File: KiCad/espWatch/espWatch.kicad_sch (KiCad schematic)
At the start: 6 parts, among them U1 Level converter, U2 NodeMCU_1.0_(ESP-12E), U3 1.8" TFT ST7735, U4 RTC DS3231

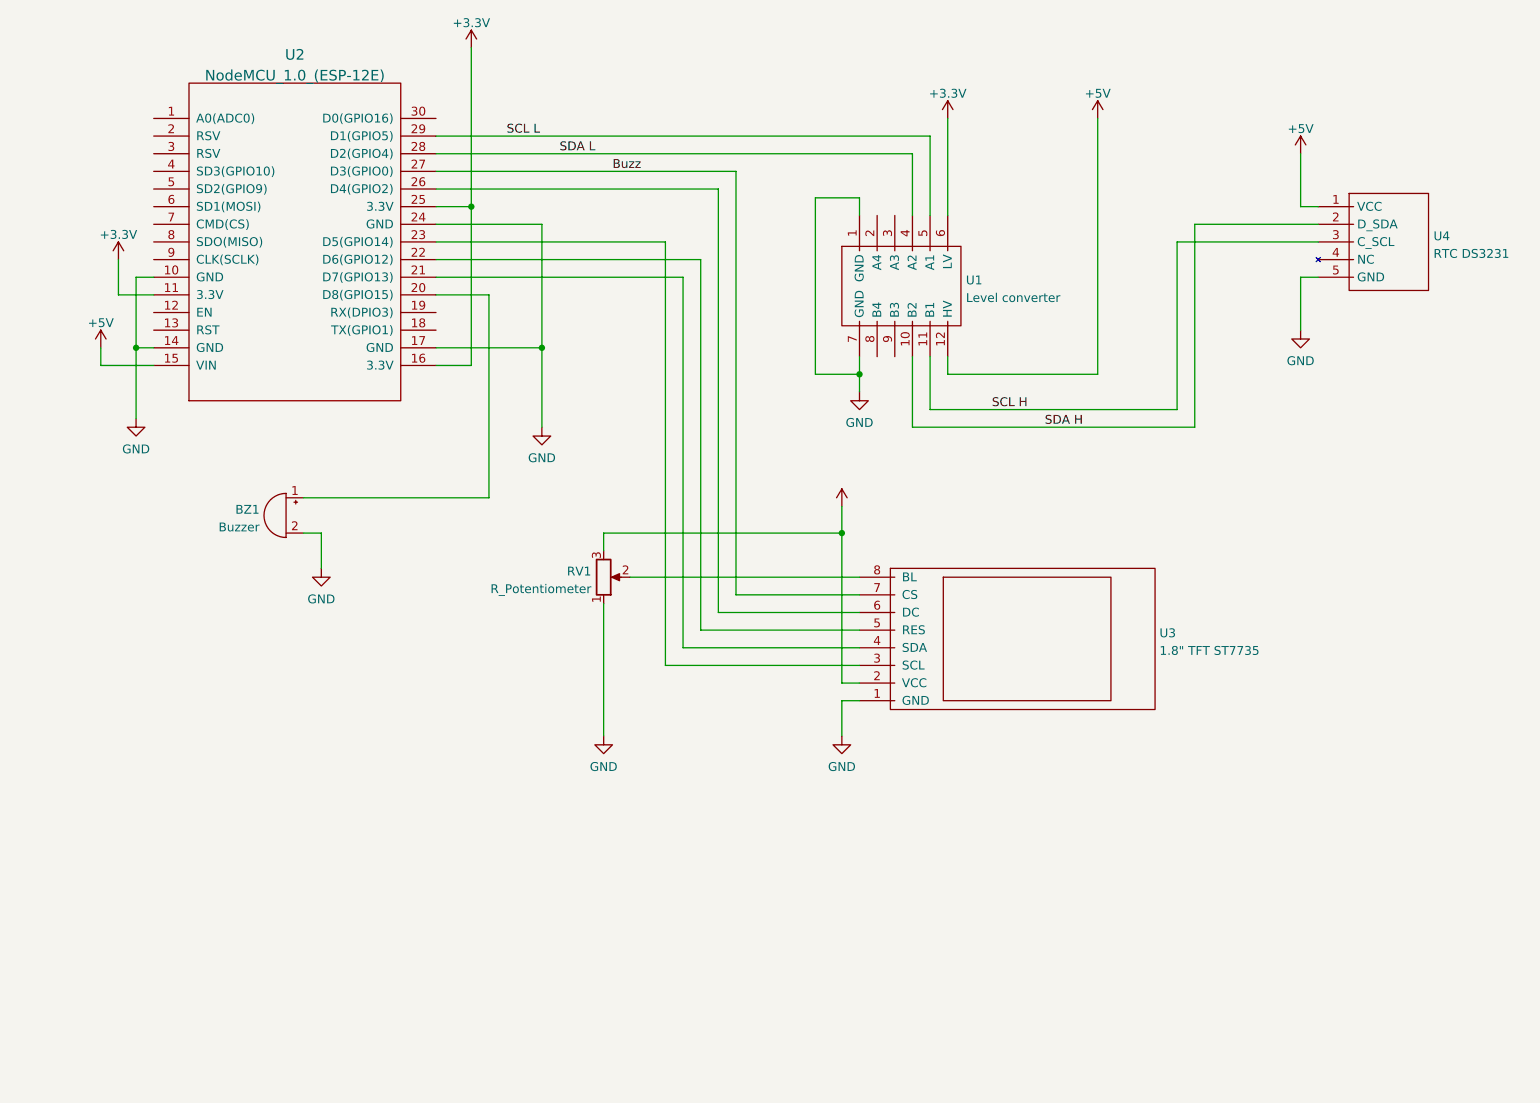
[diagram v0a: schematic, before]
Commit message: pcb and pin config
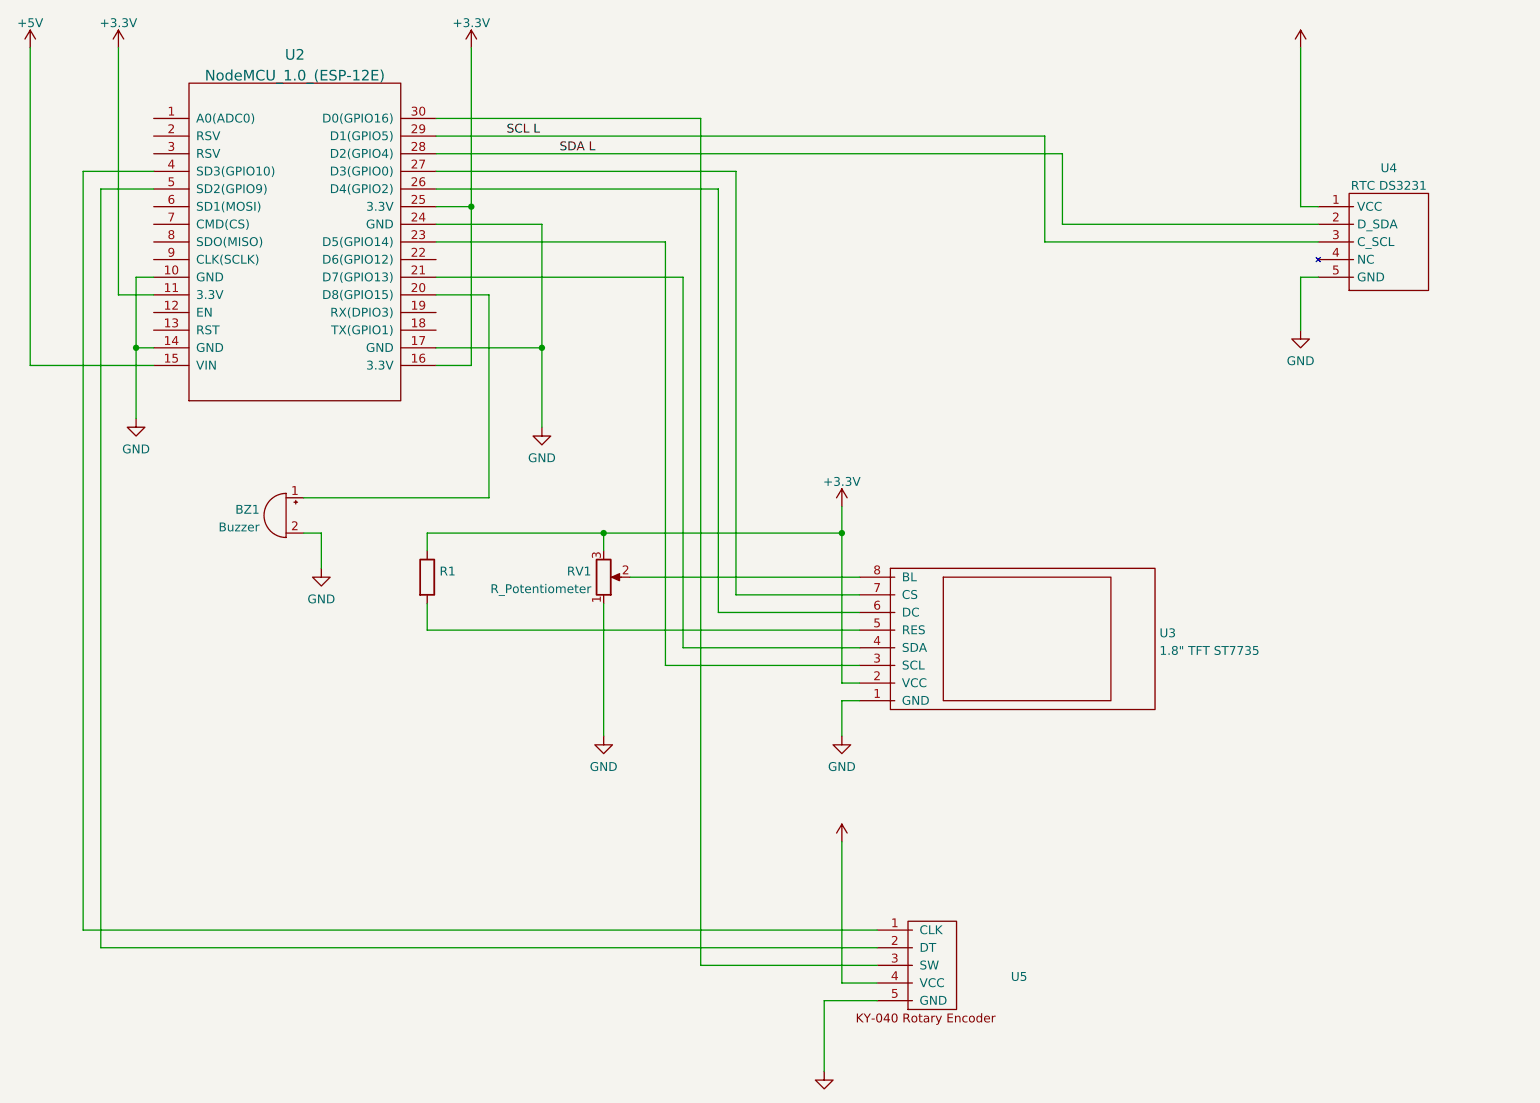
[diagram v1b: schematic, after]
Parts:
- removed U1: Level converter, My_Parts:4-channel_I2C_level_shifter_BSS138_large, symbol My_Parts:4-channel_I2C_level_shifter_BSS138
- added R1: (no value), symbol Device:R
- added U5: (no value), symbol My_Parts:KY-040_Rotary_Encoder
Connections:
- net SCL H is gone; now on net SCL L: U4.3 (C_SCL)
- net SDA H is gone; now on net SDA L: U4.2 (D_SDA)
- net +3V3: now also U4.1 (VCC), R1.1, U5.4 (VCC)
- net +5V: no longer U4.1 (VCC)
- net GND: now also U5.5 (GND)
- net at U3.5 (RES): now also R1.2; no longer U2.22 (D6(GPIO12))
- net at U2.30 (D0(GPIO16)): now also U5.3 (SW)
- net at U2.4 (SD3(GPIO10)): now also U5.1 (CLK)
- net at U2.5 (SD2(GPIO9)): now also U5.2 (DT)
- net Buzz: no longer names the net of U2.27 (D3(GPIO0)), U3.7 (CS)
